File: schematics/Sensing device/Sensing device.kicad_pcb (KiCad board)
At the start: 2 copper layers, 70.5 x 34 mm, 7 parts, among them J2 Grove_GSR, SW1 SW_Push

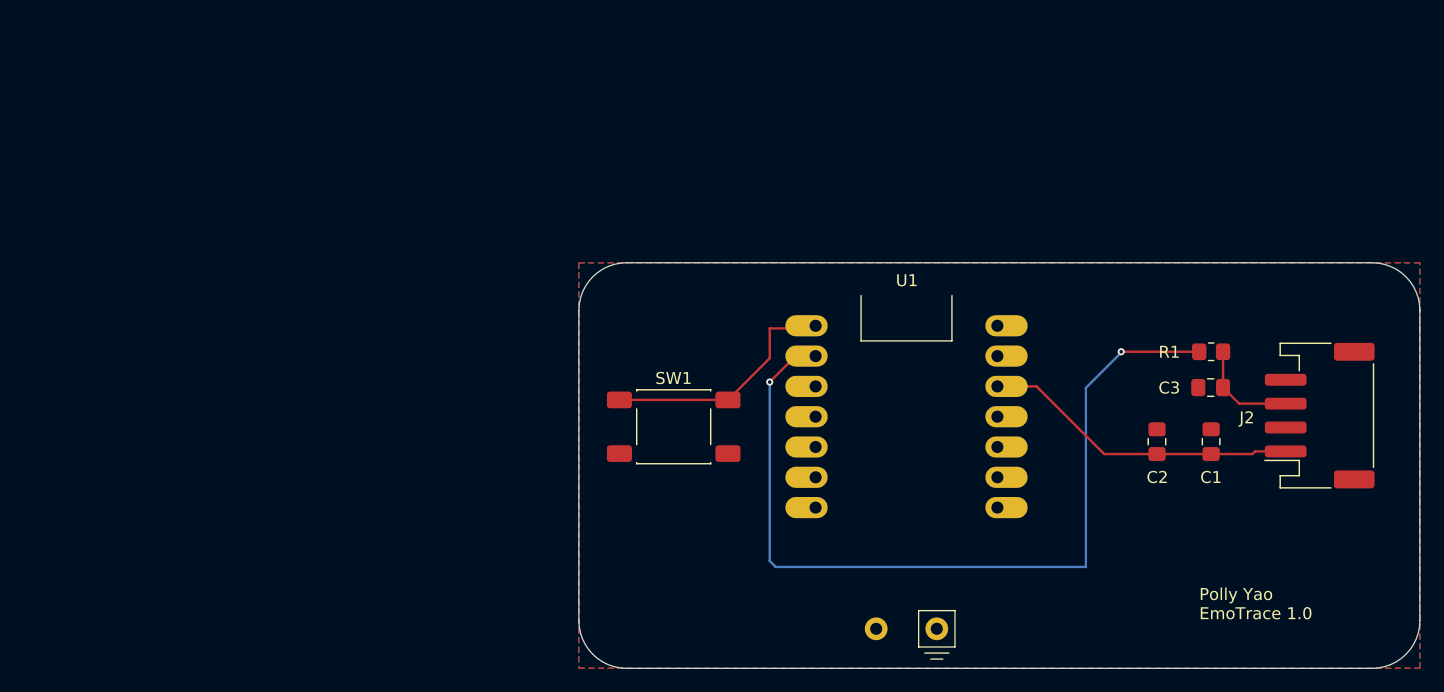
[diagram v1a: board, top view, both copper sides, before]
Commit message: kicad update
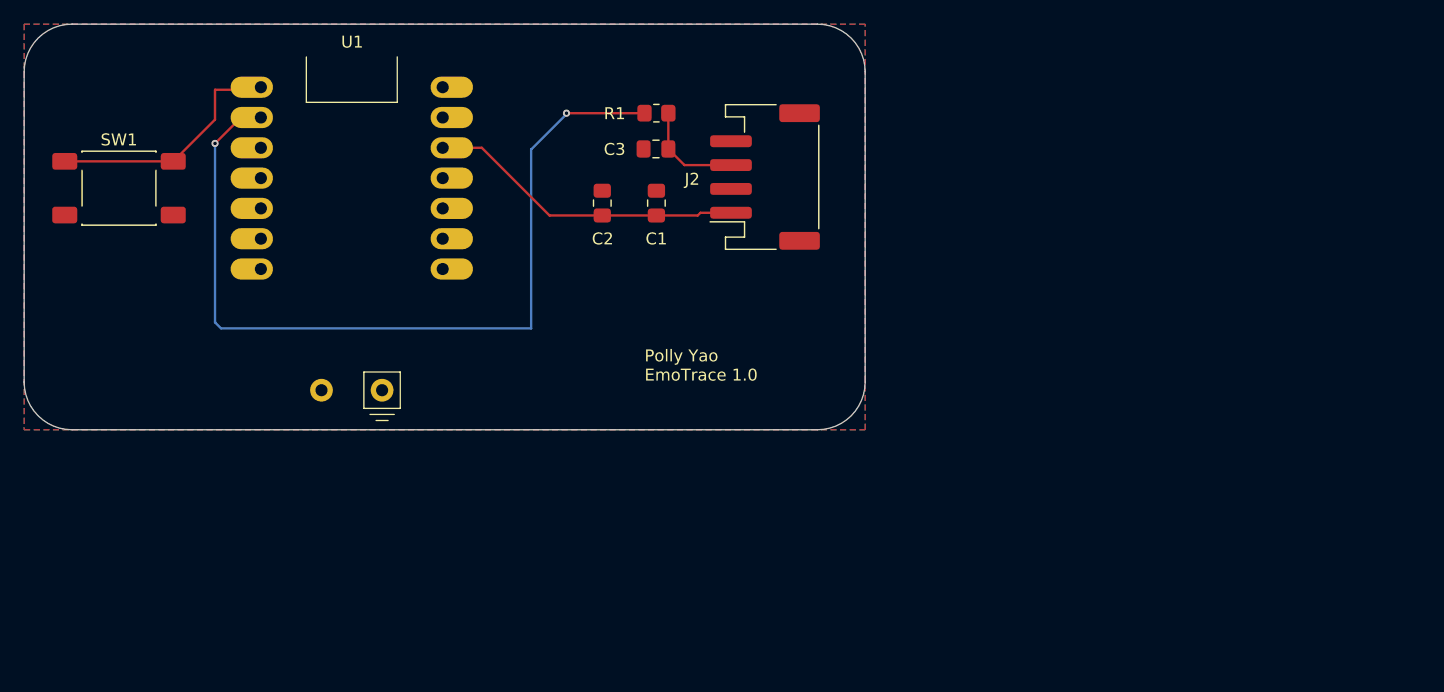
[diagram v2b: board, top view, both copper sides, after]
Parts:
- moved C1 50.6 mm to (120.5, 67.0)
- moved C2 50.6 mm to (116.0, 67.0)
- moved C3 50.6 mm to (120.5, 62.5)
- moved J2 50.6 mm to (129.6, 64.8)
- moved R1 50.6 mm to (120.5, 59.5)
- moved SW1 50.6 mm to (75.5, 65.8)
- moved U1 50.6 mm to (95.0, 64.9)
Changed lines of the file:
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@@
 		(legacy_teardrops no)
 	)
-	(paper "A4")
+	(paper "A5")
 	(title_block
-		(title "Polly Yao_EmoTrace_Display Device")
+		(title "Polly Yao_EmoTrace_Sensing Device")
 		(date "2026-02-02")
 		(rev "1.0")
@@
 	(footprint "Button_Switch_SMD:SW_Push_1P1T_NO_E-Switch_TL3301NxxxxxG"
 		(layer "F.Cu")
-		(at 121.95 85.75)
+		(at 75.45 65.75)
 		(descr "Tactile switch, 6x6 mm, H4.3 mm, gullwing terminals, https://www.e-switch.com/wp-content/uploads/2024/03/TL3301.pdf")
 		(tags "SPST button straight")
@@
 	(footprint "Capacitor_SMD:C_0805_2012Metric_Pad1.18x1.45mm_HandSolder"
 		(layer "F.Cu")
-		(at 166.9625 82.4625)
+		(at 120.4625 62.4625)
 		(descr "Capacitor SMD 0805 (2012 Metric), square (rectangular) end terminal, IPC-7351 nominal with elongated pad for handsoldering. (Body size source: IPC-SM-782 page 76, https://www.pcb-3d.com/wordpress/wp-content/uploads/ipc-sm-782a_amendment_1_and_2.pdf, https://docs.google.com/spreadsheets/d/1BsfQQcO9C6DZCsRaXUlFlo91Tg2WpOkGARC1WS5S8t0/edit?usp=sharing), generated with kicad-footprint-generator")
 		(tags "capacitor handsolder")
@@
 	(footprint "Connector_JST:JST_PH_S4B-PH-SM4-TB_1x04-1MP_P2.00mm_Horizontal"
 		(layer "F.Cu")
-		(at 176.1 84.8125 90)
+		(at 129.6 64.8125 90)
 		(descr "JST PH series connector, S4B-PH-SM4-TB (http://www.jst-mfg.com/product/pdf/eng/ePH.pdf), generated with kicad-footprint-generator")
 		(tags "connector JST PH horizontal")
@@
 	(footprint "Resistor_SMD:R_0805_2012Metric_Pad1.20x1.40mm_HandSolder"
 		(layer "F.Cu")
-		(at 167 79.4625 180)
+		(at 120.5 59.4625 180)
 		(descr "Resistor SMD 0805 (2012 Metric), square (rectangular) end terminal, IPC-7351 nominal with elongated pad for handsoldering. (Body size source: IPC-SM-782 page 72, https://www.pcb-3d.com/wordpress/wp-content/uploads/ipc-sm-782a_amendment_1_and_2.pdf), generated with kicad-footprint-generator")
 		(tags "resistor handsolder")
@@
 	(footprint "Capacitor_SMD:C_0805_2012Metric_Pad1.18x1.45mm_HandSolder"
 		(layer "F.Cu")
-		(at 167 87 90)
+		(at 120.5 67 90)
 		(descr "Capacitor SMD 0805 (2012 Metric), square (rectangular) end terminal, IPC-7351 nominal with elongated pad for handsoldering. (Body size source: IPC-SM-782 page 76, https://www.pcb-3d.com/wordpress/wp-content/uploads/ipc-sm-782a_amendment_1_and_2.pdf, https://docs.google.com/spreadsheets/d/1BsfQQcO9C6DZCsRaXUlFlo91Tg2WpOkGARC1WS5S8t0/edit?usp=sharing), generated with kicad-footprint-generator")
 		(tags "capacitor handsolder")
@@
 	(footprint "Capacitor_SMD:C_0805_2012Metric_Pad1.18x1.45mm_HandSolder"
 		(layer "F.Cu")
-		(at 162.4625 87 90)
+		(at 115.9625 67 90)
 		(descr "Capacitor SMD 0805 (2012 Metric), square (rectangular) end terminal, IPC-7351 nominal with elongated pad for handsoldering. (Body size source: IPC-SM-782 page 76, https://www.pcb-3d.com/wordpress/wp-content/uploads/ipc-sm-782a_amendment_1_and_2.pdf, https://docs.google.com/spreadsheets/d/1BsfQQcO9C6DZCsRaXUlFlo91Tg2WpOkGARC1WS5S8t0/edit?usp=sharing), generated with kicad-footprint-generator")
 		(tags "capacitor handsolder")
@@
 	(footprint "GIX_ESP32:XIAO_ESP32"
 		(layer "F.Cu")
-		(at 141.465 84.905)
+		(at 94.965 64.905)
 		(property "Reference" "U1"
 			(at 0.035 -11.405 0)
@@
 	)
 	(gr_line
-		(start 184.5 76)
-		(end 184.5 102)
+		(start 138 56)
+		(end 138 82)
 		(stroke
 			(width 0.05)
@@
 	)
 	(gr_line
-		(start 118 72)
-		(end 180.5 72)
+		(start 71.5 52)
+		(end 134 52)
 		(stroke
 			(width 0.05)
@@
 	)
 	(gr_line
-		(start 114 102)
-		(end 114 76)
+		(start 67.5 82)
+		(end 67.5 56)
 		(stroke
 			(width 0.05)
@@
 	)
 	(gr_arc
-		(start 184.5 102)
-		(mid 183.328427 104.828427)
-		(end 180.5 106)
+		(start 138 82)
+		(mid 136.828427 84.828427)
+		(end 134 86)
 		(stroke
 			(width 0.05)
@@
 	)
 	(gr_arc
-		(start 180.5 72)
-		(mid 183.328427 73.171573)
-		(end 184.5 76)
+		(start 134 52)
+		(mid 136.828427 53.171573)
+		(end 138 56)
 		(stroke
 			(width 0.05)
@@
 	)
 	(gr_arc
-		(start 118 106)
-		(mid 115.171573 104.828427)
-		(end 114 102)
+		(start 71.5 86)
+		(mid 68.671573 84.828427)
+		(end 67.5 82)
 		(stroke
 			(width 0.05)
@@
 	)
 	(gr_arc
-		(start 114 76)
-		(mid 115.171573 73.171573)
-		(end 118 72)
+		(start 67.5 56)
+		(mid 68.671573 53.171573)
+		(end 71.5 52)
 		(stroke
 			(width 0.05)
@@
 	)
 	(gr_line
-		(start 180.5 106)
-		(end 118 106)
+		(start 134 86)
+		(end 71.5 86)
 		(stroke
 			(width 0.05)
@@
 	)
 	(gr_text "Polly Yao\nEmoTrace 1.0"
-		(at 166 102 0)
+		(at 119.5 82 0)
 		(layer "F.SilkS")
 		(effects
@@
 	)
 	(segment
-		(start 173.25 87.8125)
-		(end 170.6875 87.8125)
+		(start 126.75 67.8125)
+		(end 124.1875 67.8125)
 		(width 0.2)
 		(layer "F.Cu")
@@
 	)
 	(segment
-		(start 170.4625 88.0375)
-		(end 167 88.0375)
+		(start 123.9625 68.0375)
+		(end 120.5 68.0375)
 		(width 0.2)
 		(layer "F.Cu")
@@
 	)
 	(segment
-		(start 170.6875 87.8125)
-		(end 170.4625 88.0375)
+		(start 124.1875 67.8125)
+		(end 123.9625 68.0375)
 		(width 0.2)
 		(layer "F.Cu")
@@
 	)
 	(segment
-		(start 158.0375 88.0375)
-		(end 162.4625 88.0375)
+		(start 111.5375 68.0375)
+		(end 115.9625 68.0375)
 		(width 0.2)
 		(layer "F.Cu")
@@
 	)
 	(segment
-		(start 162.4625 88.0375)
-		(end 167 88.0375)
+		(start 115.9625 68.0375)
+		(end 120.5 68.0375)
 		(width 0.2)
 		(layer "F.Cu")
@@
 	)
 	(segment
-		(start 149.085 82.365)
-		(end 152.365 82.365)
+		(start 102.585 62.365)
+		(end 105.865 62.365)
 		(width 0.2)
 		(layer "F.Cu")
@@
 	)
 	(segment
-		(start 152.365 82.365)
-		(end 158.0375 88.0375)
+		(start 105.865 62.365)
+		(end 111.5375 68.0375)
 		(width 0.2)
 		(layer "F.Cu")
@@
 	)
 	(segment
-		(start 168 79.4625)
-		(end 168 82.4625)
+		(start 121.5 59.4625)
+		(end 121.5 62.4625)
 		(width 0.2)
 		(layer "F.Cu")
@@
 	)
 	(segment
-		(start 168 82.4625)
-		(end 169.35 83.8125)
+		(start 121.5 62.4625)
+		(end 122.85 63.8125)
 		(width 0.2)
 		(layer "F.Cu")
@@
 	)
 	(segment
-		(start 169.35 83.8125)
-		(end 173.25 83.8125)
+		(start 122.85 63.8125)
+		(end 126.75 63.8125)
 		(width 0.2)
 		(layer "F.Cu")
@@
 	)
 	(segment
-		(start 132.175 79.825)
-		(end 130 82)
+		(start 85.675 59.825)
+		(end 83.5 62)
 		(width 0.2)
 		(layer "F.Cu")
@@
 	)
 	(segment
-		(start 166 79.4625)
-		(end 159.5 79.4625)
+		(start 119.5 59.4625)
+		(end 113 59.4625)
 		(width 0.2)
 		(layer "F.Cu")
@@
 	)
 	(segment
-		(start 133.845 79.825)
-		(end 132.175 79.825)
+		(start 87.345 59.825)
+		(end 85.675 59.825)
 		(width 0.2)
 		(layer "F.Cu")
@@
 	)
 	(segment
-		(start 159.5 79.4625)
-		(end 159.4625 79.4625)
+		(start 113 59.4625)
+		(end 112.9625 59.4625)
 		(width 0.2)
 		(layer "F.Cu")
@@
 	)
 	(via
-		(at 159.4625 79.4625)
+		(at 112.9625 59.4625)
 		(size 0.6)
 		(drill 0.3)
@@
 	)
 	(via
-		(at 130 82)
+		(at 83.5 62)
 		(size 0.6)
 		(drill 0.3)
@@
 	)
 	(segment
-		(start 130.5 97.5)
-		(end 156.5 97.5)
+		(start 84 77.5)
+		(end 110 77.5)
 		(width 0.2)
 		(layer "B.Cu")
@@
 	)
 	(segment
-		(start 130 97)
-		(end 130.5 97.5)
+		(start 83.5 77)
+		(end 84 77.5)
 		(width 0.2)
 		(layer "B.Cu")
@@
 	)
 	(segment
-		(start 156.5 97.5)
-		(end 156.5 82.5)
+		(start 110 77.5)
+		(end 110 62.5)
 		(width 0.2)
 		(layer "B.Cu")
@@
 	)
 	(segment
-		(start 130 82)
-		(end 130 97)
+		(start 83.5 62)
+		(end 83.5 77)
 		(width 0.2)
 		(layer "B.Cu")
@@
 	)
 	(segment
-		(start 156.5 82.5)
-		(end 159.5 79.5)
+		(start 110 62.5)
+		(end 113 59.5)
 		(width 0.2)
 		(layer "B.Cu")
@@
 	)
 	(segment
-		(start 117.4 83.5)
-		(end 126.5 83.5)
+		(start 70.9 63.5)
+		(end 80 63.5)
 		(width 0.2)
 		(layer "F.Cu")
@@
 	)
 	(segment
-		(start 133.63 77.5)
-		(end 133.845 77.285)
+		(start 87.13 57.5)
+		(end 87.345 57.285)
 		(width 0.2)
 		(layer "F.Cu")
@@
 	)
 	(segment
-		(start 130 80)
-		(end 130 77.5)
+		(start 83.5 60)
+		(end 83.5 57.5)
 		(width 0.2)
 		(layer "F.Cu")
@@
 	)
 	(segment
-		(start 126.5 83.5)
-		(end 130 80)
+		(start 80 63.5)
+		(end 83.5 60)
 		(width 0.2)
 		(layer "F.Cu")
@@
 	)
 	(segment
-		(start 130 77.5)
-		(end 133.63 77.5)
+		(start 83.5 57.5)
+		(end 87.13 57.5)
 		(width 0.2)
 		(layer "F.Cu")
@@
 		(polygon
 			(pts
-				(xy 114 72) (xy 114 106) (xy 184.5 106) (xy 184.5 72)
-			)
-		)
+				(xy 67.5 52) (xy 67.5 86) (xy 138 86) (xy 138 52)
+			)
+		)
